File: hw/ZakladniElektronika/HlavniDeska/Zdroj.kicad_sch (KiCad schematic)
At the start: 12 parts, among them U3 BQ298012

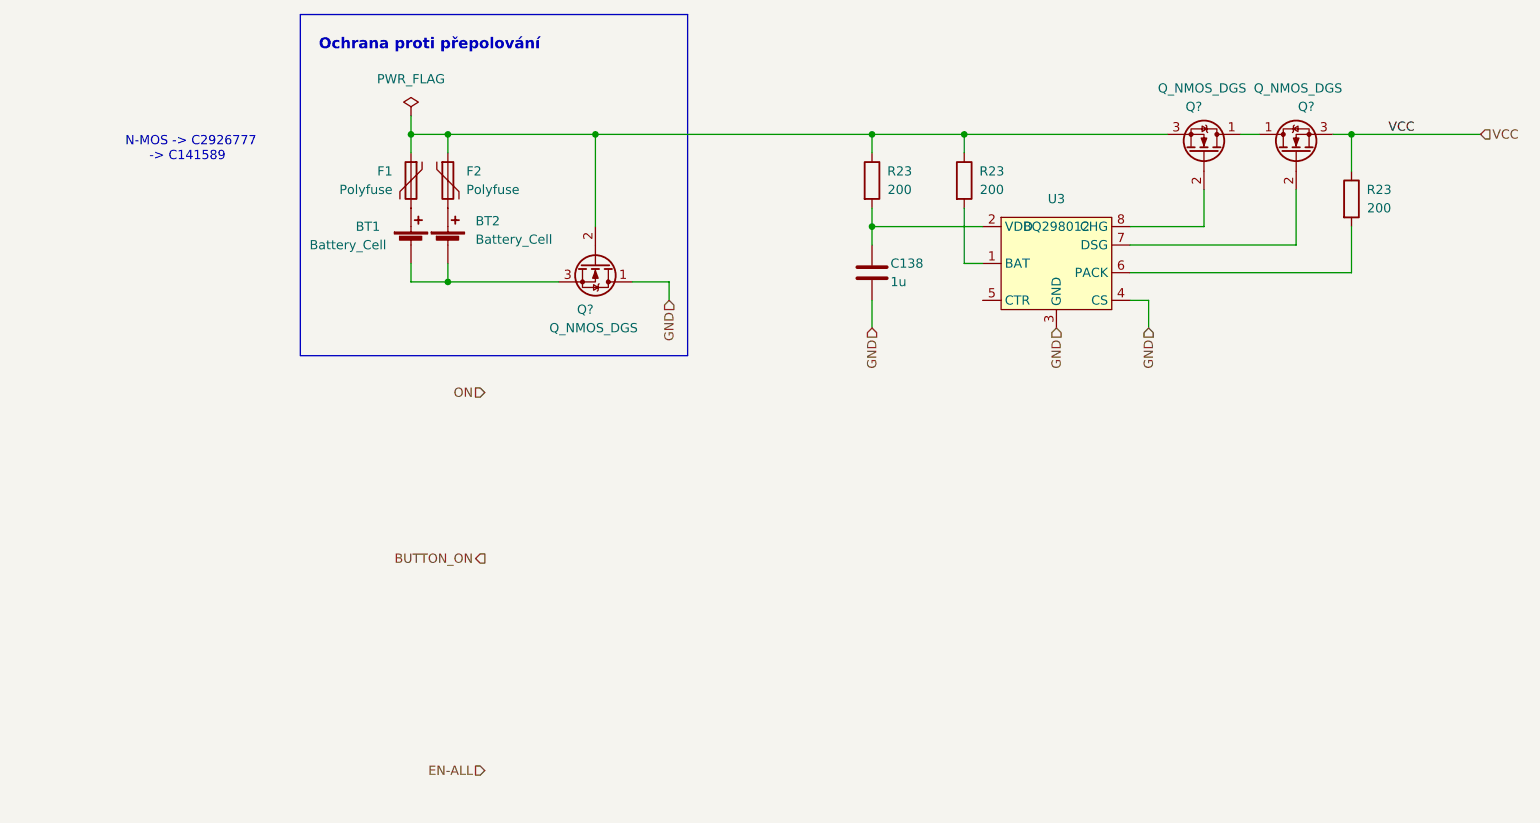
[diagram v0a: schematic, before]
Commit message: Zavazbení zapínání
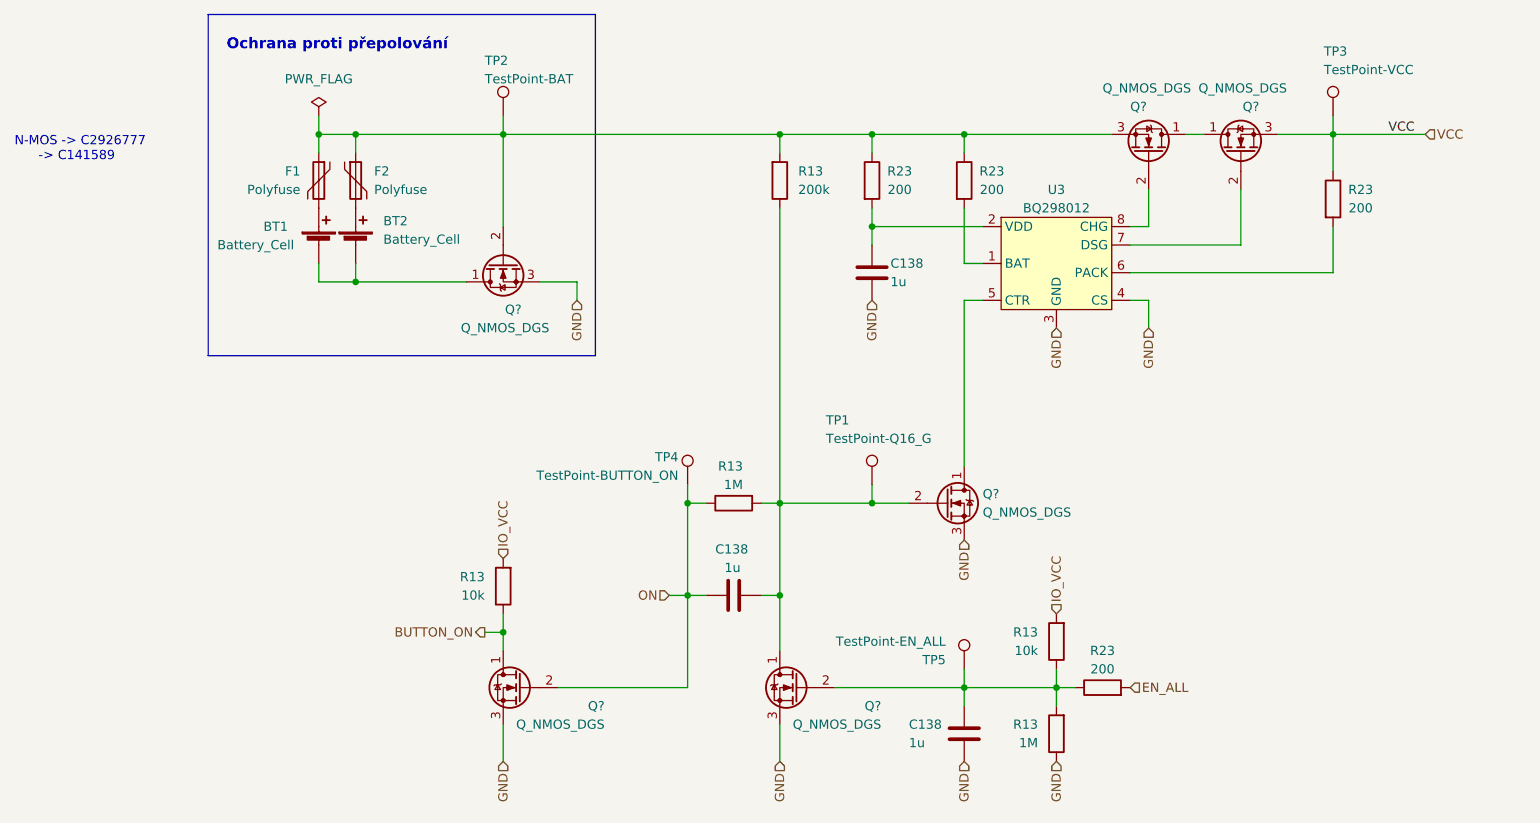
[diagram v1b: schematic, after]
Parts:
- removed Q? (x2): Q_NMOS_DGS, symbol Device:Q_NMOS_DGS
- added C138 (x2): 1u, Resistor_SMD:R_0402_1005Metric, symbol Device:C
- added Q? (x2): Q_NMOS_DGS, symbol Device:Q_NMOS_DGS
- added Q? (x3): Q_NMOS_DGS, Package_TO_SOT_SMD:SOT-23, symbol Device:Q_NMOS_DGS
- added R13 (x2): 10k, Resistor_SMD:R_0402_1005Metric, symbol Device:R
- added R13: 200k, Resistor_SMD:R_0402_1005Metric, symbol Device:R
- added R13 (x2): 1M, Resistor_SMD:R_0402_1005Metric, symbol Device:R
- added R23: 200, Resistor_SMD:R_0402_1005Metric, symbol Device:R
- added TP1: TestPoint-Q16_G, symbol Connector:TestPoint
- added TP2: TestPoint-BAT, symbol Connector:TestPoint
- added TP3: TestPoint-VCC, symbol Connector:TestPoint
- added TP4: TestPoint-BUTTON_ON, symbol Connector:TestPoint
- added TP5: TestPoint-EN_ALL, symbol Connector:TestPoint
- Q?: Basic/Extended (none) -> E; LCSC (none) -> C2926777
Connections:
- net BUTTON_ON: now also Q?.1 (D), R13.1
- net GND: now also Q?.3 (S), C138.2, Q?.3 (S), Q?.3 (S), Q?.3 (S), R13.1; no longer Q?.1 (D)
- net ON: now also C138.2, Q?.2 (G), R13.1, TP4.1
- net VCC: now also Q?.3 (S), TP3.1
- net at F1.1, F2.1, Q?.2 (G)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: now also Q?.3 (S), R13.2, TP2.1
- net at U3.7 (DSG): now also Q?.2 (G)
- net at BT1.2 (-), BT2.2 (-): now also Q?.1 (D); no longer Q?.3 (S)
- net at U3.8 (CHG): now also Q?.2 (G)
- net at U3.5 (CTR): now also Q?.1 (D)
- new net: Q?.1 (D), Q?.1 (D)
- new net: C138.1, Q?.2 (G), R13.1, R13.2, R23.1, TP5.1
- new net: C138.1, Q?.1 (D), Q?.2 (G), R13.1, R13.2, TP1.1
- new net EN_ALL: R23.2
- new net IO_VCC: R13.2, R13.2
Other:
- moved on the sheet: BT1, BT2, F1, F2, Q?, R23
